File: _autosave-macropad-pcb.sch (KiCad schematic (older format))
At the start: 24 parts, among them SW1 SW_Push, U1 ATmega32U4-AU, Y1 16MHz

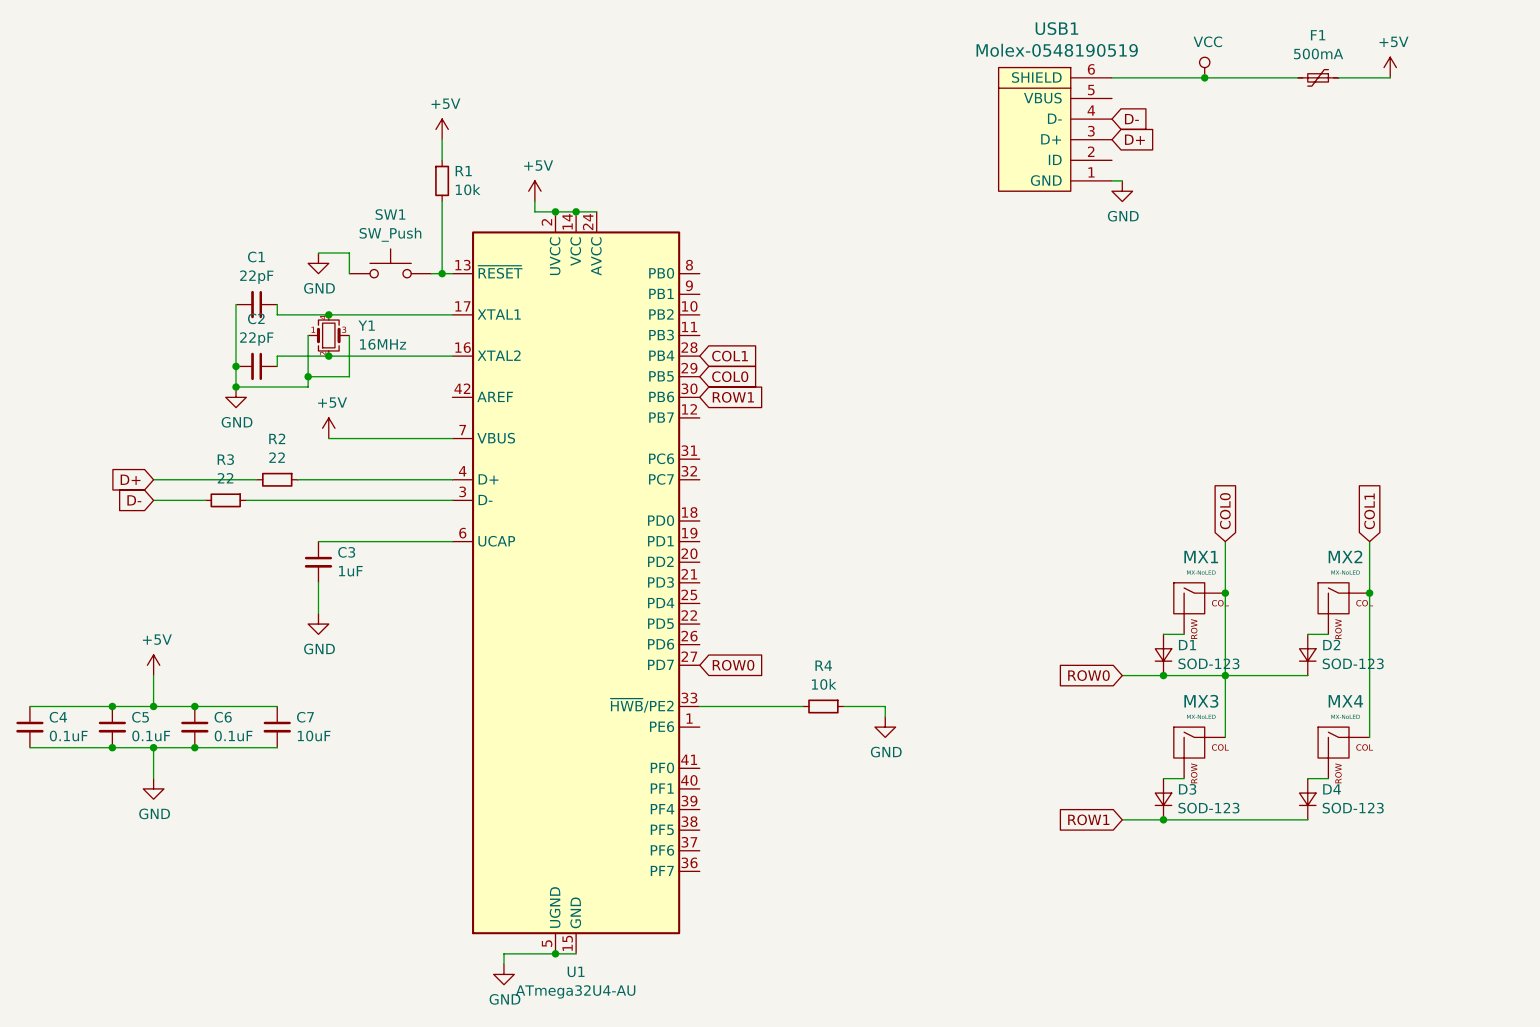
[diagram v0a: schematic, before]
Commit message: pcb saves
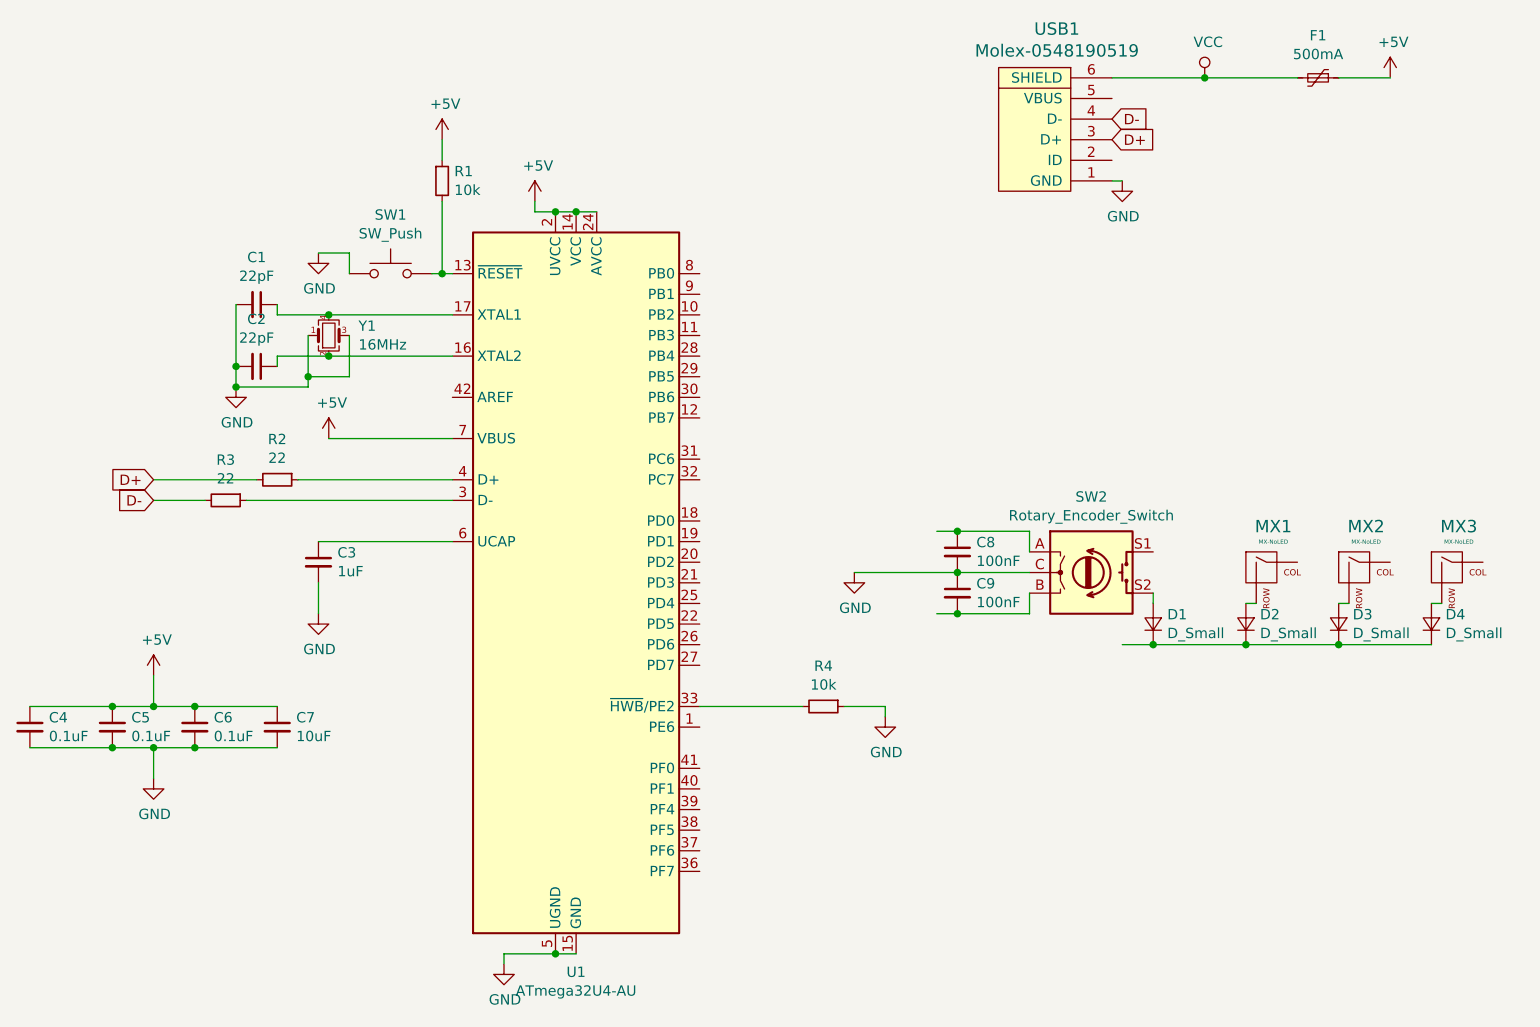
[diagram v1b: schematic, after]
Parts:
- removed MX4: MX-NoLED, symbol MX_Alps_Hybrid:MX-NoLED
- added C8, C9: 100nF, Capacitor_SMD:C_0805_2012Metric, symbol Device:C_Small
- added SW2: Rotary_Encoder_Switch, symbol Device:Rotary_Encoder_Switch
- D1, D2, D3, D4: value SOD-123 -> D_Small
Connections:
- net labels removed: COL0, COL1, ROW0, ROW1
- wire segments 64 -> 66
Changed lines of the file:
@@
 	8400 2000 8350 2000
 $Comp
-L MX_Alps_Hybrid:MX-NoLED MX1
-U 1 1 5F291437
-P 8750 4050
-F 0 "MX1" H 8783 4273 60  0000 C CNN
-F 1 "MX-NoLED" H 8783 4199 20  0000 C CNN
-F 2 "" H 8125 4025 60  0001 C CNN
-F 3 "" H 8125 4025 60  0001 C CNN
-	1    8750 4050
+L Device:Rotary_Encoder_Switch SW2
+U 1 1 5F25C130
+P 8250 3900
+F 0 "SW2" H 8250 4267 50  0000 C CNN
+F 1 "Rotary_Encoder_Switch" H 8250 4176 50  0000 C CNN
+F 2 "" H 8100 4060 50  0001 C CNN
+F 3 "~" H 8250 4160 50  0001 C CNN
+	1    8250 3900
 	1    0    0    -1
 $EndComp
 $Comp
-L Device:D_Small D1
-U 1 1 5F2925B5
-P 8600 4300
-F 0 "D1" V 8646 4232 50  0000 R CNN
-F 1 "SOD-123" V 8555 4232 50  0000 R CNN
-F 2 "Diode_SMD:D_SOD-123" V 8600 4300 50  0001 C CNN
-F 3 "~" V 8600 4300 50  0001 C CNN
-	1    8600 4300
+L MX_Alps_Hybrid:MX-NoLED MX1
+U 1 1 5F26C0EC
+P 9100 3900
+F 0 "MX1" H 9133 4123 60  0000 C CNN
+F 1 "MX-NoLED" H 9133 4049 20  0000 C CNN
+F 2 "" H 8475 3875 60  0001 C CNN
+F 3 "" H 8475 3875 60  0001 C CNN
+	1    9100 3900
+	1    0    0    -1
+$EndComp
+$Comp
+L MX_Alps_Hybrid:MX-NoLED MX2
+U 1 1 5F26CAFC
+P 9550 3900
+F 0 "MX2" H 9583 4123 60  0000 C CNN
+F 1 "MX-NoLED" H 9583 4049 20  0000 C CNN
+F 2 "" H 8925 3875 60  0001 C CNN
+F 3 "" H 8925 3875 60  0001 C CNN
+	1    9550 3900
+	1    0    0    -1
+$EndComp
+$Comp
+L MX_Alps_Hybrid:MX-NoLED MX3
+U 1 1 5F26D0BB
+P 10000 3900
+F 0 "MX3" H 10033 4123 60  0000 C CNN
+F 1 "MX-NoLED" H 10033 4049 20  0000 C CNN
+F 2 "" H 9375 3875 60  0001 C CNN
+F 3 "" H 9375 3875 60  0001 C CNN
+	1    10000 3900
+	1    0    0    -1
+$EndComp
+Wire Wire Line
+	9050 4050 9000 4050
+Wire Wire Line
+	9500 4050 9450 4050
+Wire Wire Line
+	9950 4050 9900 4050
+$Comp
+L Device:D_Small D2
+U 1 1 5F27215D
+P 9000 4150
+F 0 "D2" V 9046 4082 50  0000 R CNN
+F 1 "D_Small" V 8955 4082 50  0000 R CNN
+F 2 "Diode_SMD:D_SOD-123" V 9000 4150 50  0001 C CNN
+F 3 "~" V 9000 4150 50  0001 C CNN
+	1    9000 4150
+	0    -1   -1   0
+$EndComp
+$Comp
+L Device:D_Small D3
+U 1 1 5F273088
+P 9450 4150
+F 0 "D3" V 9496 4082 50  0000 R CNN
+F 1 "D_Small" V 9405 4082 50  0000 R CNN
+F 2 "Diode_SMD:D_SOD-123" V 9450 4150 50  0001 C CNN
+F 3 "~" V 9450 4150 50  0001 C CNN
+	1    9450 4150
+	0    -1   -1   0
+$EndComp
+$Comp
+L Device:D_Small D4
+U 1 1 5F273732
+P 9900 4150
+F 0 "D4" V 9946 4082 50  0000 R CNN
+F 1 "D_Small" V 9855 4082 50  0000 R CNN
+F 2 "Diode_SMD:D_SOD-123" V 9900 4150 50  0001 C CNN
+F 3 "~" V 9900 4150 50  0001 C CNN
+	1    9900 4150
 	0    -1   -1   0
 $EndComp
 Wire Wire Line
-	8600 4200 8700 4200
+	9000 4250 9450 4250
+Connection ~ 9450 4250
+Wire Wire Line
+	9450 4250 9900 4250
 $Comp
-L MX_Alps_Hybrid:MX-NoLED MX2
-U 1 1 5F29D570
-P 9450 4050
-F 0 "MX2" H 9483 4273 60  0000 C CNN
-F 1 "MX-NoLED" H 9483 4199 20  0000 C CNN
-F 2 "" H 8825 4025 60  0001 C CNN
-F 3 "" H 8825 4025 60  0001 C CNN
-	1    9450 4050
+L Device:D_Small D1
+U 1 1 5F2760A0
+P 8550 4150
+F 0 "D1" V 8596 4082 50  0000 R CNN
+F 1 "D_Small" V 8505 4082 50  0000 R CNN
+F 2 "Diode_SMD:D_SOD-123" V 8550 4150 50  0001 C CNN
+F 3 "~" V 8550 4150 50  0001 C CNN
+	1    8550 4150
+	0    -1   -1   0
+$EndComp
+Wire Wire Line
+	7950 3700 7950 3800
+Wire Wire Line
+	7950 4000 7950 4100
+$Comp
+L power:GND #PWR0114
+U 1 1 5F28B8F7
+P 7100 3900
+F 0 "#PWR0114" H 7100 3650 50  0001 C CNN
+F 1 "GND" H 7105 3727 50  0000 C CNN
+F 2 "" H 7100 3900 50  0001 C CNN
+F 3 "" H 7100 3900 50  0001 C CNN
+	1    7100 3900
 	1    0    0    -1
 $EndComp
 $Comp
-L Device:D_Small D2
-U 1 1 5F29D576
-P 9300 4300
-F 0 "D2" V 9346 4232 50  0000 R CNN
-F 1 "SOD-123" V 9255 4232 50  0000 R CNN
-F 2 "Diode_SMD:D_SOD-123" V 9300 4300 50  0001 C CNN
-F 3 "~" V 9300 4300 50  0001 C CNN
-	1    9300 4300
-	0    -1   -1   0
-$EndComp
-Wire Wire Line
-	9300 4200 9400 4200
-$Comp
-L MX_Alps_Hybrid:MX-NoLED MX3
-U 1 1 5F29F40F
-P 8750 4750
-F 0 "MX3" H 8783 4973 60  0000 C CNN
-F 1 "MX-NoLED" H 8783 4899 20  0000 C CNN
-F 2 "" H 8125 4725 60  0001 C CNN
-F 3 "" H 8125 4725 60  0001 C CNN
-	1    8750 4750
+L Device:C_Small C9
+U 1 1 5F28C3AA
+P 7600 4000
+F 0 "C9" H 7692 4046 50  0000 L CNN
+F 1 "100nF" H 7692 3955 50  0000 L CNN
+F 2 "Capacitor_SMD:C_0805_2012Metric" H 7600 4000 50  0001 C CNN
+F 3 "~" H 7600 4000 50  0001 C CNN
+	1    7600 4000
 	1    0    0    -1
 $EndComp
 $Comp
-L Device:D_Small D3
-U 1 1 5F29F415
-P 8600 5000
-F 0 "D3" V 8646 4932 50  0000 R CNN
-F 1 "SOD-123" V 8555 4932 50  0000 R CNN
-F 2 "Diode_SMD:D_SOD-123" V 8600 5000 50  0001 C CNN
-F 3 "~" V 8600 5000 50  0001 C CNN
-	1    8600 5000
-	0    -1   -1   0
-$EndComp
-Wire Wire Line
-	8600 4900 8700 4900
-$Comp
-L MX_Alps_Hybrid:MX-NoLED MX4
-U 1 1 5F2A1394
-P 9450 4750
-F 0 "MX4" H 9483 4973 60  0000 C CNN
-F 1 "MX-NoLED" H 9483 4899 20  0000 C CNN
-F 2 "" H 8825 4725 60  0001 C CNN
-F 3 "" H 8825 4725 60  0001 C CNN
-	1    9450 4750
+L Device:C_Small C8
+U 1 1 5F28D003
+P 7600 3800
+F 0 "C8" H 7692 3846 50  0000 L CNN
+F 1 "100nF" H 7692 3755 50  0000 L CNN
+F 2 "Capacitor_SMD:C_0805_2012Metric" H 7600 3800 50  0001 C CNN
+F 3 "~" H 7600 3800 50  0001 C CNN
+	1    7600 3800
 	1    0    0    -1
 $EndComp
-$Comp
-L Device:D_Small D4
-U 1 1 5F2A139A
-P 9300 5000
-F 0 "D4" V 9346 4932 50  0000 R CNN
-F 1 "SOD-123" V 9255 4932 50  0000 R CNN
-F 2 "Diode_SMD:D_SOD-123" V 9300 5000 50  0001 C CNN
-F 3 "~" V 9300 5000 50  0001 C CNN
-	1    9300 5000
-	0    -1   -1   0
-$EndComp
+Connection ~ 7600 3900
 Wire Wire Line
-	9300 4900 9400 4900
+	7600 3900 7950 3900
 Wire Wire Line
-	9300 4400 8900 4400
-Connection ~ 8600 4400
+	7500 4100 7600 4100
+Connection ~ 7600 4100
 Wire Wire Line
-	8600 4400 8400 4400
+	7600 4100 7950 4100
 Wire Wire Line
-	9300 5100 8600 5100
-Connection ~ 8600 5100
+	7950 3700 7600 3700
+Connection ~ 7600 3700
 Wire Wire Line
-	8600 5100 8400 5100
+	7500 3700 7600 3700
 Wire Wire Line
-	8900 3750 8900 4000
+	8550 4000 8550 4050
+Connection ~ 9000 4250
+Connection ~ 8550 4250
 Wire Wire Line
-	8900 4000 8900 4400
-Connection ~ 8900 4000
-Connection ~ 8900 4400
+	8550 4250 9000 4250
 Wire Wire Line
-	8900 4400 8600 4400
+	8400 4250 8550 4250
 Wire Wire Line
-	9600 4700 9600 4000
-Connection ~ 9600 4000
-Wire Wire Line
-	9600 4000 9600 3750
-Text GLabel 8900 3750 1    50   Input ~ 0
-COL0
-Text GLabel 9600 3750 1    50   Input ~ 0
-COL1
-Text GLabel 8400 4400 0    50   Input ~ 0
-ROW0
-Text GLabel 8400 5100 0    50   Input ~ 0
-ROW1
-Text GLabel 6350 2950 2    50   Input ~ 0
-COL0
-Text GLabel 6350 2850 2    50   Input ~ 0
-COL1
-Text GLabel 6350 4350 2    50   Input ~ 0
-ROW0
-Text GLabel 6350 3050 2    50   Input ~ 0
-ROW1
-Wire Wire Line
-	8900 4400 8900 4700
+	7100 3900 7600 3900
 $EndSCHEMATC
